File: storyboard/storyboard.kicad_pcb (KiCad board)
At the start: 2 copper layers, 284.7 x 94.2 mm, 169 parts, among them J1 Debug Breakout, J2 Pico-EZmate, J3 MICROMOD-2222-C, J4 Conn_02x20_Odd_Even, J5 M2.5 Standoff, SW1 Switch_1u, SW10 Switch_1u, SW11 Switch_1u, SW12 Switch_1u, SW13 Switch_1u, SW14 Switch_1u, SW15 Switch_1u, SW16 Switch_1u, SW17 Switch_1u, SW18 Switch_1u, SW19 Switch_1u, SW2 Switch_1u, SW20 Switch_1u, SW21 Switch_1u, SW22 Switch_1u, SW23 Switch_1u, SW24 Switch_1u, SW25 Switch_1u, SW26 Switch_1u, SW27 Switch_1u, SW28 Switch_1u, SW29 Switch_1u, SW3 Switch_1u, SW30 Switch_1u, SW31 Switch_1u, SW32 Switch_1u, SW33 Switch_1u, SW34 Switch_1u, SW35 Switch_1u, SW36 Switch_1u, SW37 Switch_1u, SW38 Switch_1u, SW39 Switch_1u, SW4 Switch_1u, SW40 Switch_1u, SW41 Switch_1u, SW42 Switch_1u, SW43 Switch_1u, SW44 Switch_1u, SW45 Switch_1u, SW46 Switch_1u, SW47 Switch_1u, SW48 Switch_1u, SW49 Switch_1u, SW5 Switch_1u, SW50 Switch_1u, SW51 Switch_1u, SW52 Switch_1u, SW53 Switch_1u, SW54 Switch_1u, SW55 Switch_1u, SW56 Switch_1u, SW57 Switch_1u, SW58 Switch_1u, SW59 Switch_1u, SW6 Switch_1u, SW60 Switch_1u, SW61 RESET, SW62 BOOT, SW7 Switch_1u, SW8 Switch_1u, SW9 Switch_1u, U1 74HC164 (SIPO), U2 74HC165 (PISO), U3 74HC165 (PISO), U4 AP7361C-33E

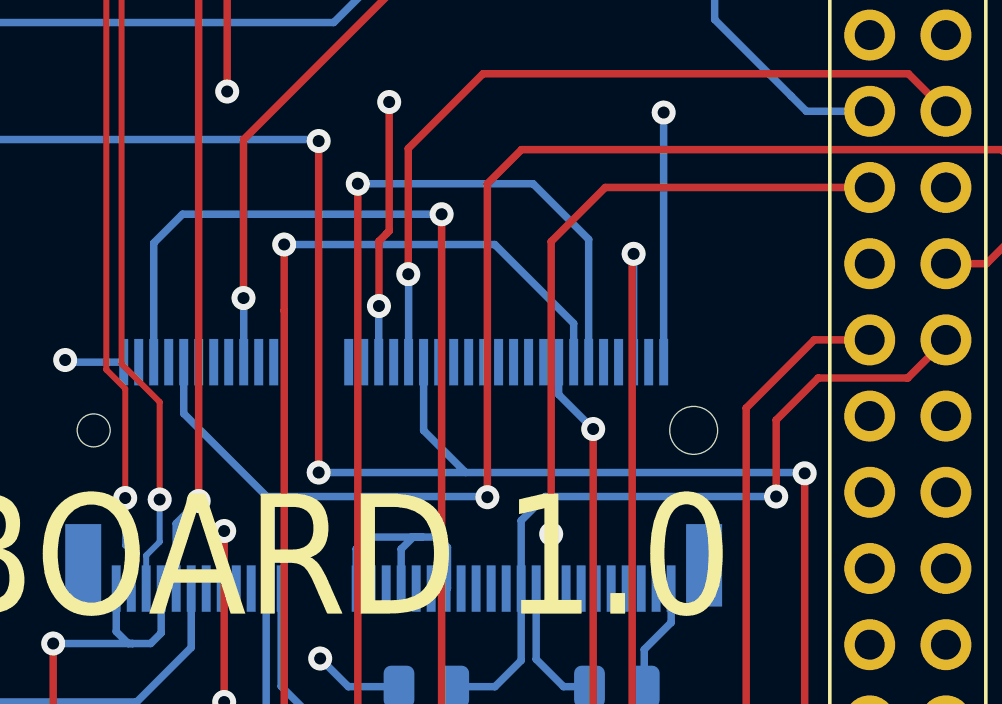
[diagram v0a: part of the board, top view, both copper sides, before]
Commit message: update latest production files
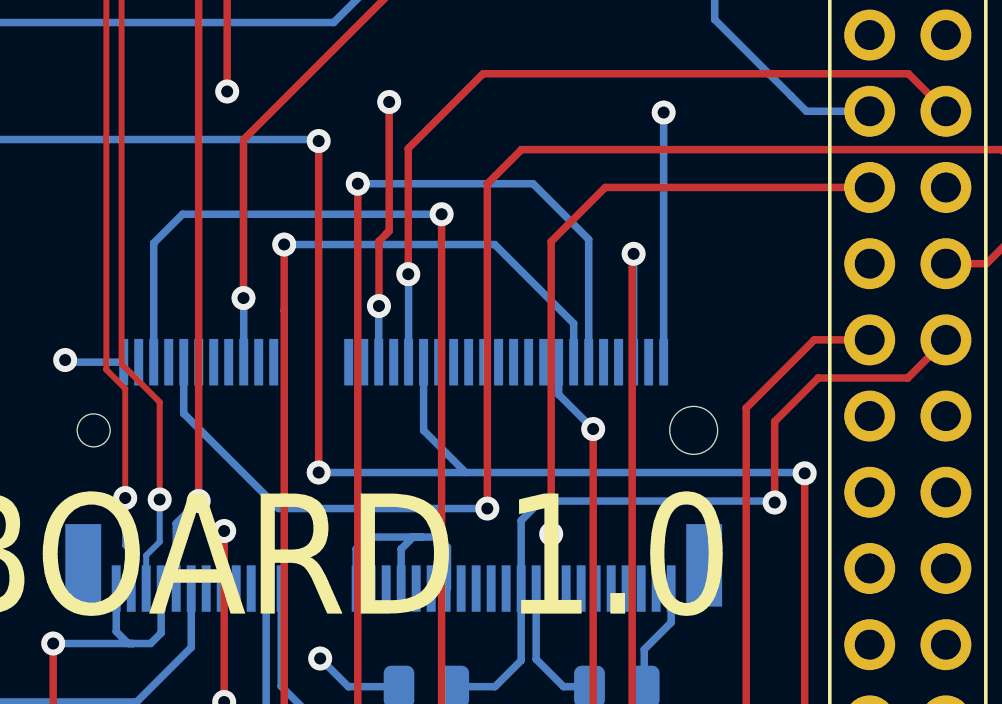
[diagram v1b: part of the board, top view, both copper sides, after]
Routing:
- net DISPLAY_DC: track 47.2 -> 47.7 mm
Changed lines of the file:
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@@
       (layerselection 0x00010fc_ffffffff)
       (disableapertmacros false)
-      (usegerberextensions false)
-      (usegerberattributes true)
-      (usegerberadvancedattributes true)
-      (creategerberjobfile true)
+      (usegerberextensions true)
+      (usegerberattributes false)
+      (usegerberadvancedattributes false)
+      (creategerberjobfile false)
       (svguseinch false)
       (svgprecision 6)
@@
       (psa4output false)
       (plotreference true)
-      (plotvalue true)
+      (plotvalue false)
       (plotinvisibletext false)
       (sketchpadsonfab false)
-      (subtractmaskfromsilk false)
+      (subtractmaskfromsilk true)
       (outputformat 1)
       (mirror false)
       (drillshape 0)
       (scaleselection 1)
-      (outputdirectory "../production_files/gerber/")
+      (outputdirectory "../production_files/pcb-gerbers/")
     )
   )
@@
     (fp_line (start -10.94994 1.24968) (end -10.94994 -5.24764) (layer "Dwgs.User") (width 0.1524))
     (fp_line (start 10.94994 1.24968) (end 9.4996 1.24968) (layer "Dwgs.User") (width 0.1524))
-    (fp_arc (start 11.000756 19.247478) (mid 10.700626 19.948301) (end 9.99998 20.24888) (layer "Dwgs.User") (width 0.04826))
+    (fp_arc (start 11.000756 19.247478) (mid 10.70062 19.948306) (end 9.99998 20.24888) (layer "Dwgs.User") (width 0.04826))
     (fp_arc (start 10.396526 2.249096) (mid 10.062741 2.090116) (end 9.92378 1.74752) (layer "Dwgs.User") (width 0.0508))
     (fp_arc (start -9.999214 20.246359) (mid -10.69834 19.947022) (end -10.9982 19.24812) (layer "Dwgs.User") (width 0.04826))
@@
   (segment (start 202.25224 89.98424) (end 202.25224 91.218235) (width 0.2) (layer "B.Cu") (net 86))
   (segment (start 202.051424 88.2) (end 202.051424 89.783424) (width 0.2) (layer "B.Cu") (net 86))
+  (segment (start 214.122 77.724) (end 215.258801 76.587199) (width 0.25) (layer "F.Cu") (net 89))
+  (segment (start 214.122 88.55) (end 214.122 77.724) (width 0.25) (layer "F.Cu") (net 89))
+  (segment (start 231.273199 76.587199) (end 232.156 77.47) (width 0.25) (layer "F.Cu") (net 89))
   (segment (start 232.156 78.994) (end 230.762 80.388) (width 0.25) (layer "F.Cu") (net 89))
   (segment (start 232.156 77.47) (end 232.156 78.994) (width 0.25) (layer "F.Cu") (net 89))
-  (segment (start 214.122 88.172) (end 214.122 77.724) (width 0.25) (layer "F.Cu") (net 89))
   (segment (start 215.258801 76.587199) (end 231.273199 76.587199) (width 0.25) (layer "F.Cu") (net 89))
-  (segment (start 214.122 77.724) (end 215.258801 76.587199) (width 0.25) (layer "F.Cu") (net 89))
   (segment (start 230.762 80.388) (end 229.408 80.388) (width 0.25) (layer "F.Cu") (net 89))
-  (segment (start 231.273199 76.587199) (end 232.156 77.47) (width 0.25) (layer "F.Cu") (net 89))
-  (via (at 214.122 88.172) (size 0.8) (drill 0.4) (layers "F.Cu" "B.Cu") (net 89))
-  (segment (start 214.1 88.15) (end 206.768 88.15) (width 0.25) (layer "B.Cu") (net 89))
+  (via (at 214.122 88.55) (size 0.8) (drill 0.4) (layers "F.Cu" "B.Cu") (net 89))
   (segment (start 204.0023 85.3843) (end 204.0023 83.671895) (width 0.25) (layer "B.Cu") (net 89))
-  (segment (start 206.768 88.15) (end 204.0023 85.3843) (width 0.25) (layer "B.Cu") (net 89))
-  (segment (start 214.122 88.172) (end 214.1 88.15) (width 0.25) (layer "B.Cu") (net 89))
+  (segment (start 214.122 88.55) (end 207.168 88.55) (width 0.25) (layer "B.Cu") (net 89))
+  (segment (start 207.168 88.55) (end 204.0023 85.3843) (width 0.25) (layer "B.Cu") (net 89))
   (segment (start 194.056 122.936) (end 194.056 94.996) (width 0.25) (layer "F.Cu") (net 90))
   (via (at 194.056 94.996) (size 0.8) (drill 0.4) (layers "F.Cu" "B.Cu") (net 90))
@@
   (segment (start 211.486595 80.738755) (end 211.49784 80.75) (width 0.25) (layer "B.Cu") (net 106))
   (segment (start 211.49784 80.75) (end 211.49784 83.671895) (width 0.25) (layer "B.Cu") (net 106))
-  (segment (start 223.75 88.15) (end 223.75 85.6) (width 0.25) (layer "F.Cu") (net 119))
-  (segment (start 223.75 85.6) (end 225.15 84.2) (width 0.25) (layer "F.Cu") (net 119))
-  (segment (start 225.15 84.2) (end 228.136 84.2) (width 0.25) (layer "F.Cu") (net 119))
+  (segment (start 223.7 88.35) (end 223.7 85.65) (width 0.25) (layer "F.Cu") (net 119))
   (segment (start 228.136 84.2) (end 229.408 82.928) (width 0.25) (layer "F.Cu") (net 119))
-  (via (at 223.75 88.15) (size 0.8) (drill 0.4) (layers "F.Cu" "B.Cu") (net 119))
-  (segment (start 216.05 88.15) (end 215.24942 88.95058) (width 0.25) (layer "B.Cu") (net 119))
+  (segment (start 225.15 84.2) (end 228.136 84.2) (width 0.25) (layer "F.Cu") (net 119))
+  (segment (start 223.7 85.65) (end 225.15 84.2) (width 0.25) (layer "F.Cu") (net 119))
+  (via (at 223.7 88.35) (size 0.8) (drill 0.4) (layers "F.Cu" "B.Cu") (net 119))
+  (segment (start 215.24942 88.95058) (end 215.24942 91.218235) (width 0.25) (layer "B.Cu") (net 119))
   (segment (start 214.376 94.488) (end 215.24942 93.61458) (width 0.25) (layer "B.Cu") (net 119))
-  (segment (start 223.75 88.15) (end 216.05 88.15) (width 0.25) (layer "B.Cu") (net 119))
   (segment (start 215.24942 93.61458) (end 215.24942 91.218235) (width 0.25) (layer "B.Cu") (net 119))
-  (segment (start 215.24942 88.95058) (end 215.24942 91.218235) (width 0.25) (layer "B.Cu") (net 119))
+  (segment (start 215.9 88.3) (end 215.24942 88.95058) (width 0.25) (layer "B.Cu") (net 119))
+  (segment (start 223.7 88.35) (end 223.65 88.3) (width 0.25) (layer "B.Cu") (net 119))
   (segment (start 213.0025 94.488) (end 214.376 94.488) (width 0.25) (layer "B.Cu") (net 119))
+  (segment (start 223.65 88.3) (end 215.9 88.3) (width 0.25) (layer "B.Cu") (net 119))
   (segment (start 222.8 96.3) (end 222.75 96.25) (width 0.25) (layer "F.Cu") (net 121))
   (segment (start 222.75 96.25) (end 222.75 85.2) (width 0.25) (layer "F.Cu") (net 121))
